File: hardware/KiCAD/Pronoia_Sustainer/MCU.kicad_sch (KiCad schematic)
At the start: 21 parts, among them J11 640457-2, J12 Conn_01x24_Pin, J14 Conn_01x24_Pin, Q5 AO3400A, Q6 AO3400A, U2 Teensy4.1

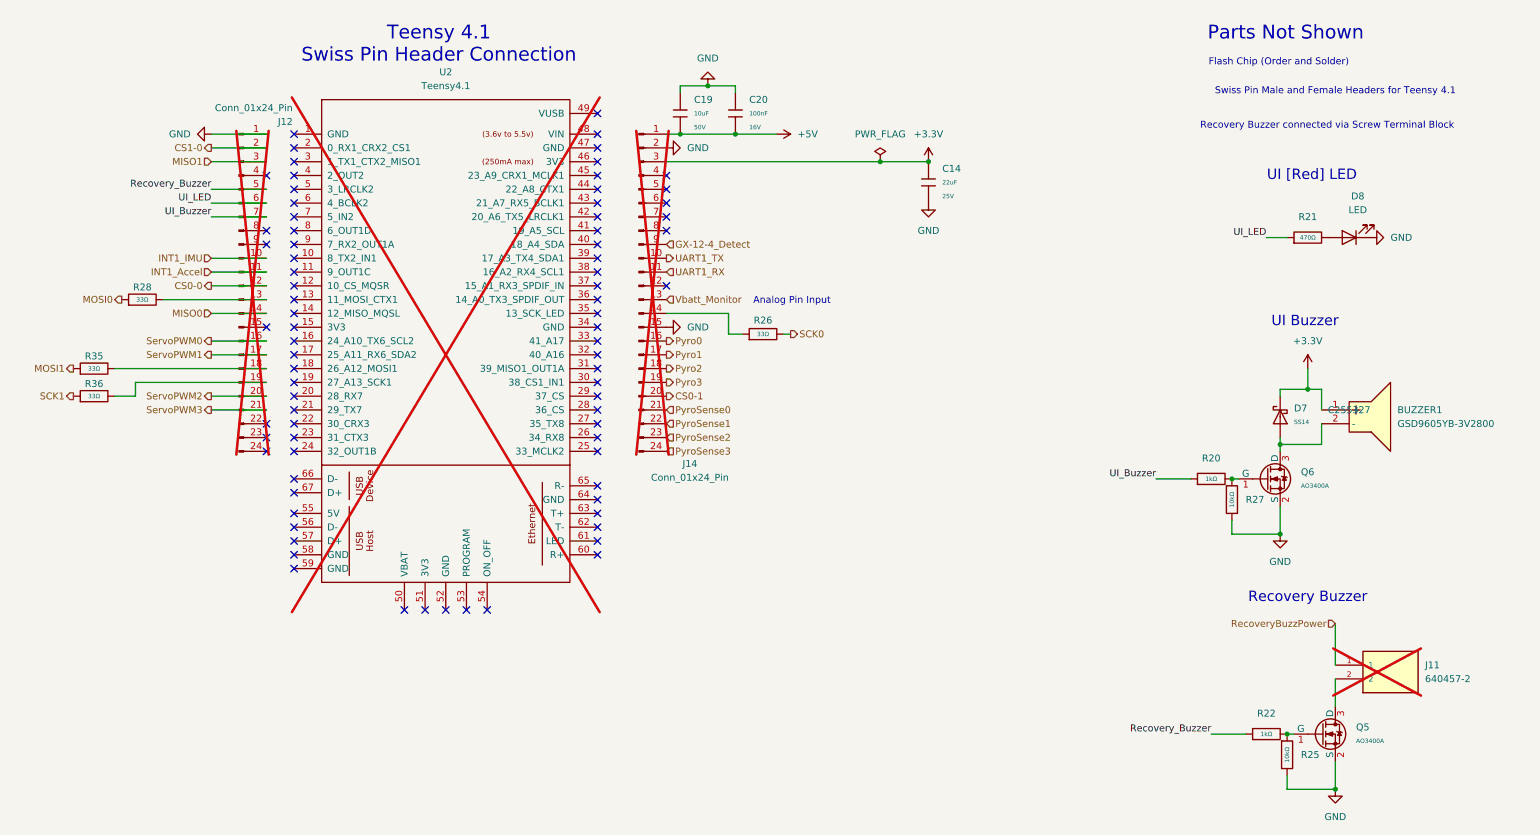
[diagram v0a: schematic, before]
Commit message: Updated codebase
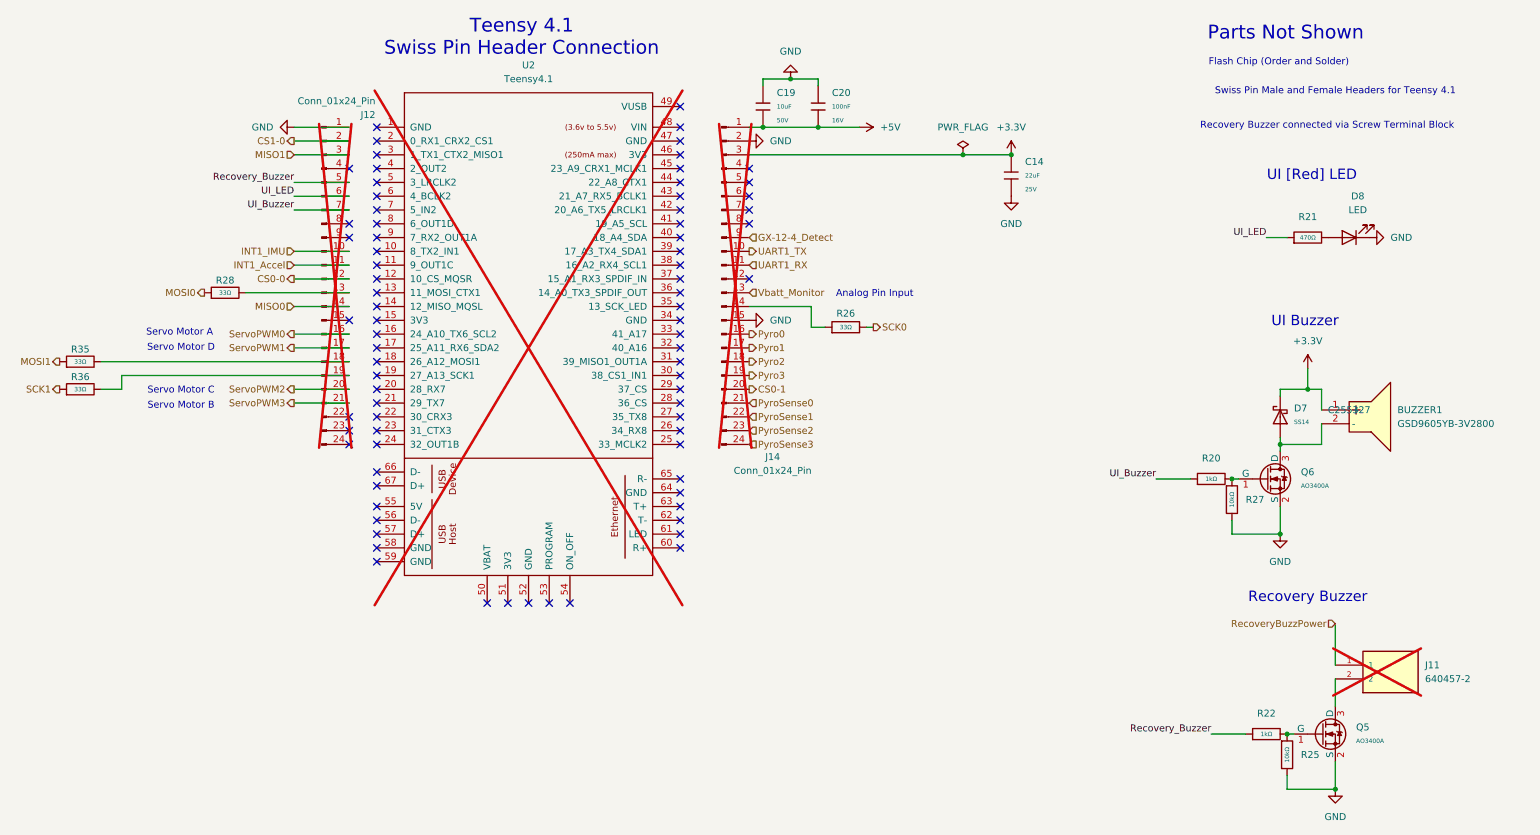
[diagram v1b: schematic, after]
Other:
- note added: "Servo Motor A"
- note added: "Servo Motor B"
- note added: "Servo Motor C"
- note added: "Servo Motor D"
- moved on the sheet: C14, C19, C20, J12, J14, R26, R28, R35, R36, U2
